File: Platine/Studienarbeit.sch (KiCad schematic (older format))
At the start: 47 parts, among them Y1 8MHz

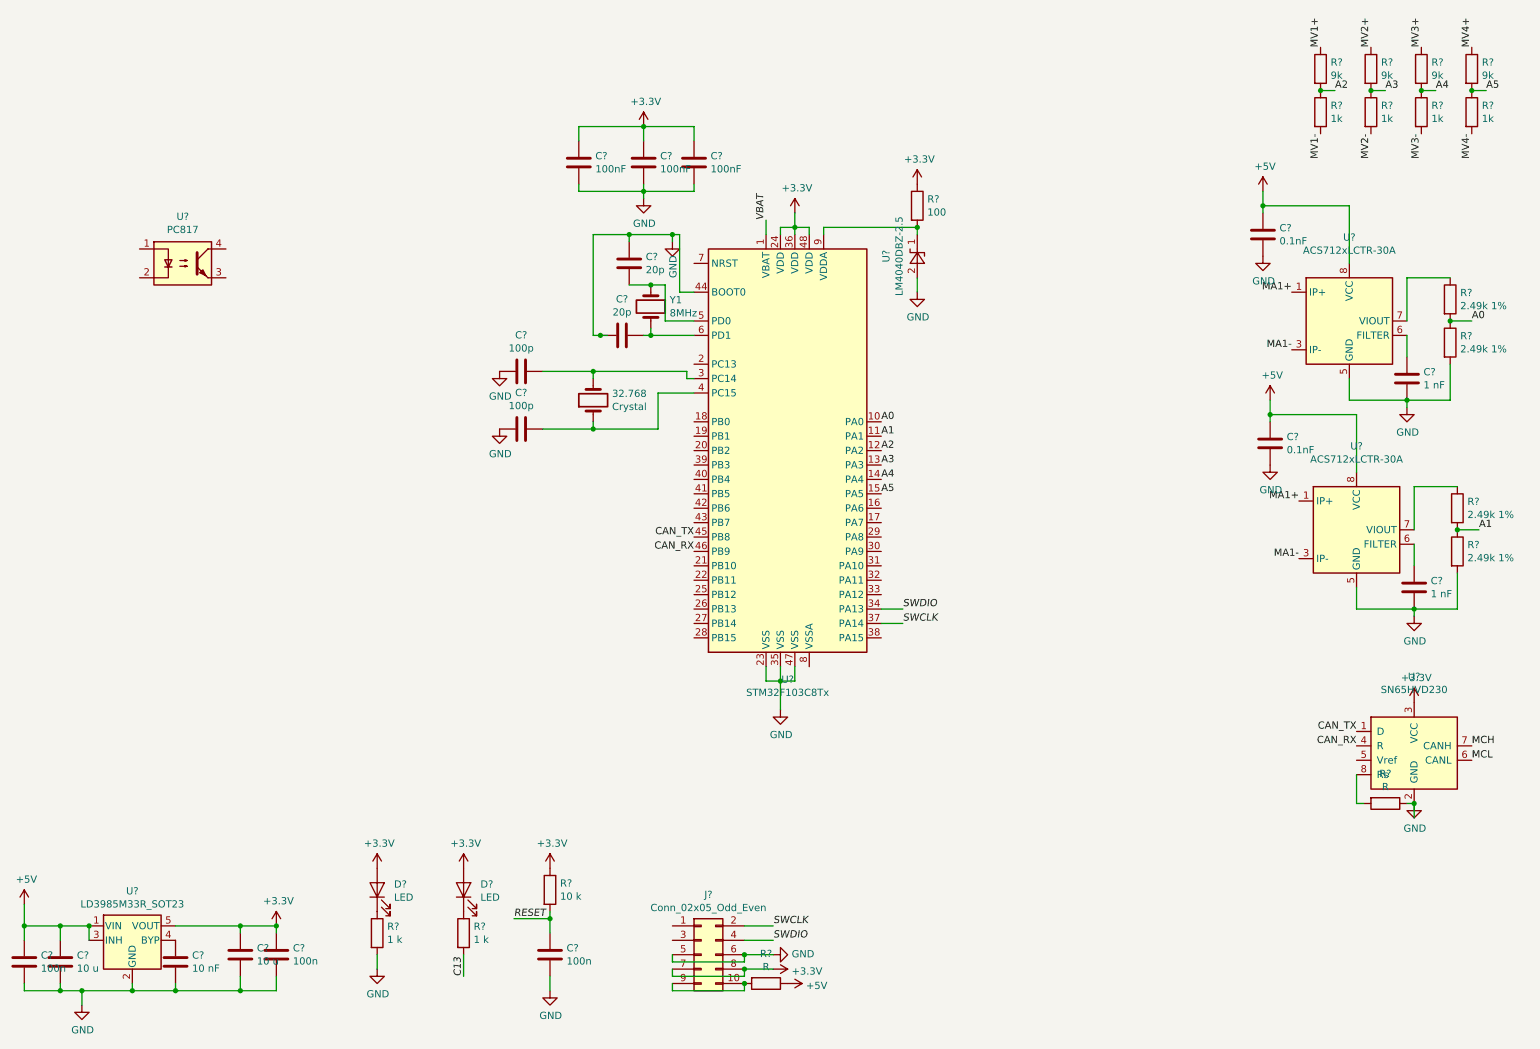
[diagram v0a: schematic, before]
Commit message: To much for description
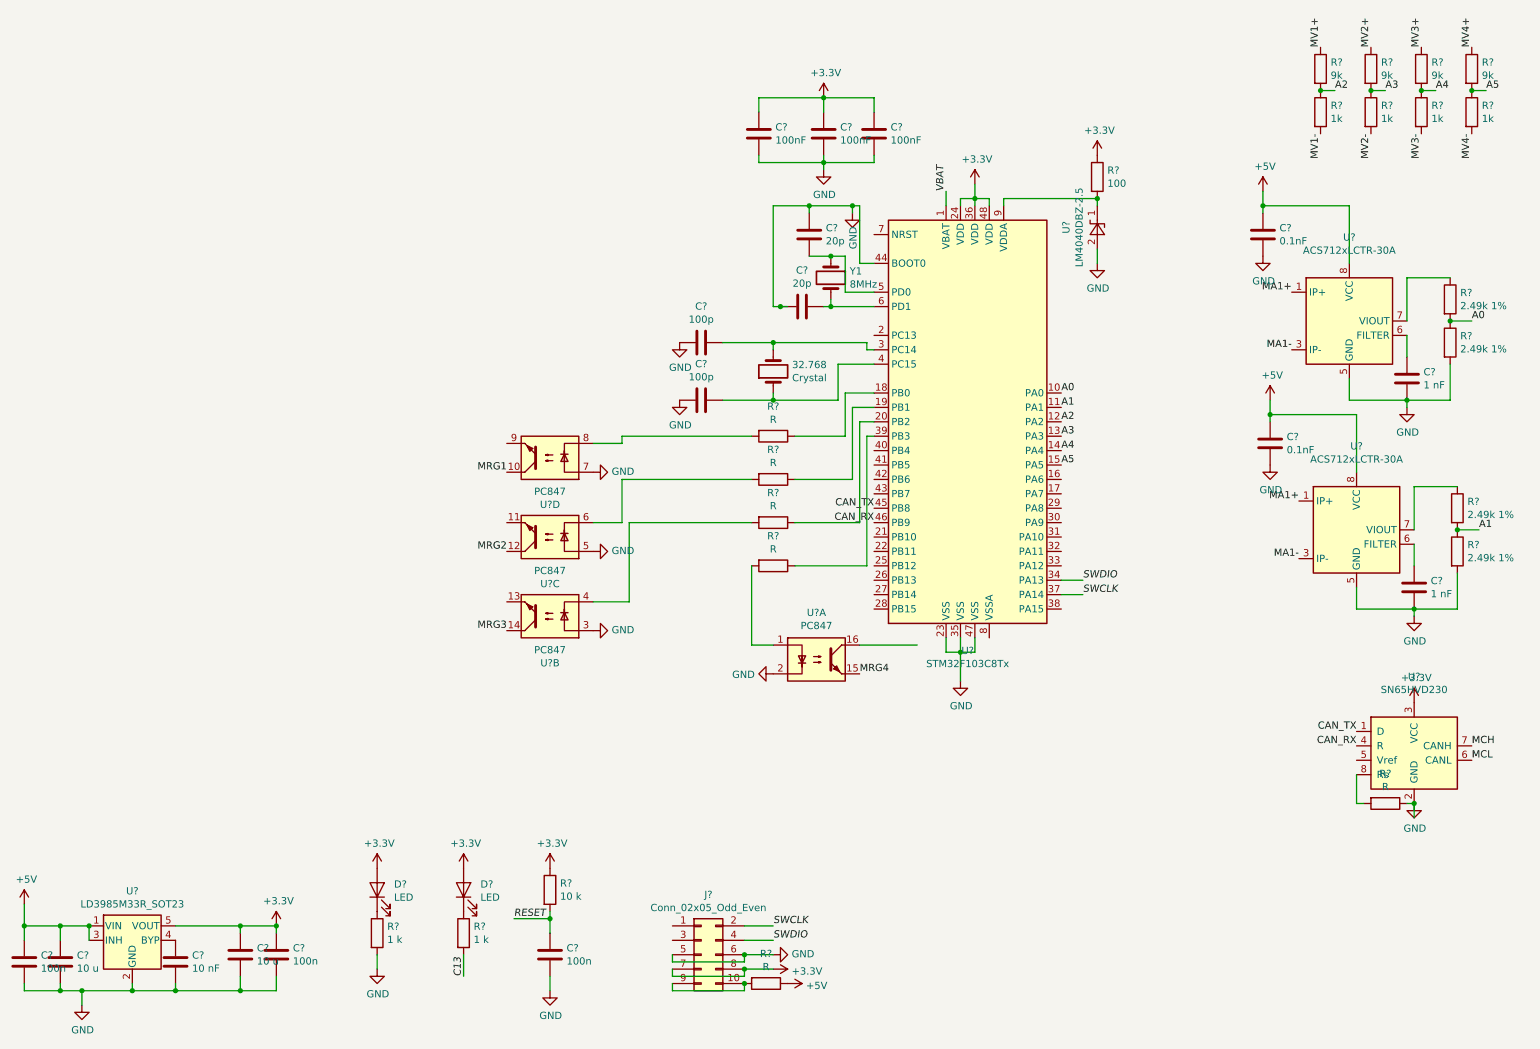
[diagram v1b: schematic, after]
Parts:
- removed U?: PC817, Package_DIP:DIP-4_W7.62mm, symbol Isolator:PC817
- added R? (x4): R, symbol Device:R
- added U? (x4): PC847, Package_DIP:DIP-16_W7.62mm, symbol Isolator:PC847
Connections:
- net GND: now also U?.2, U?.3, U?.5, U?.7
- net at U?.18 (PB0): now also R?.1
- net at U?.19 (PB1): now also R?.1
- net at U?.20 (PB2): now also R?.1
- net at U?.39 (PB3): now also R?.1
- new net: R?.2, U?.8
- new net: R?.2, U?.6
- new net: R?.2, U?.4
- new net: R?.2, U?.1
- new net MRG1: U?.10
- new net MRG2: U?.12
- new net MRG3: U?.14
- new net MRG4: U?.15
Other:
- moved on the sheet: 32.768, C?, R?, U?, Y1
